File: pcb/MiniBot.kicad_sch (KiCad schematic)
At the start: 39 parts, among them IC1 MMC5633NJL, IC2 MIC23050-SYML-TR, J1 Conn_01x08, J2 Conn_01x02, J3 GSB1C41110SSHR, U1 ESP32-C3-MINI-1-H4X, U3 MCP73832-2-OT

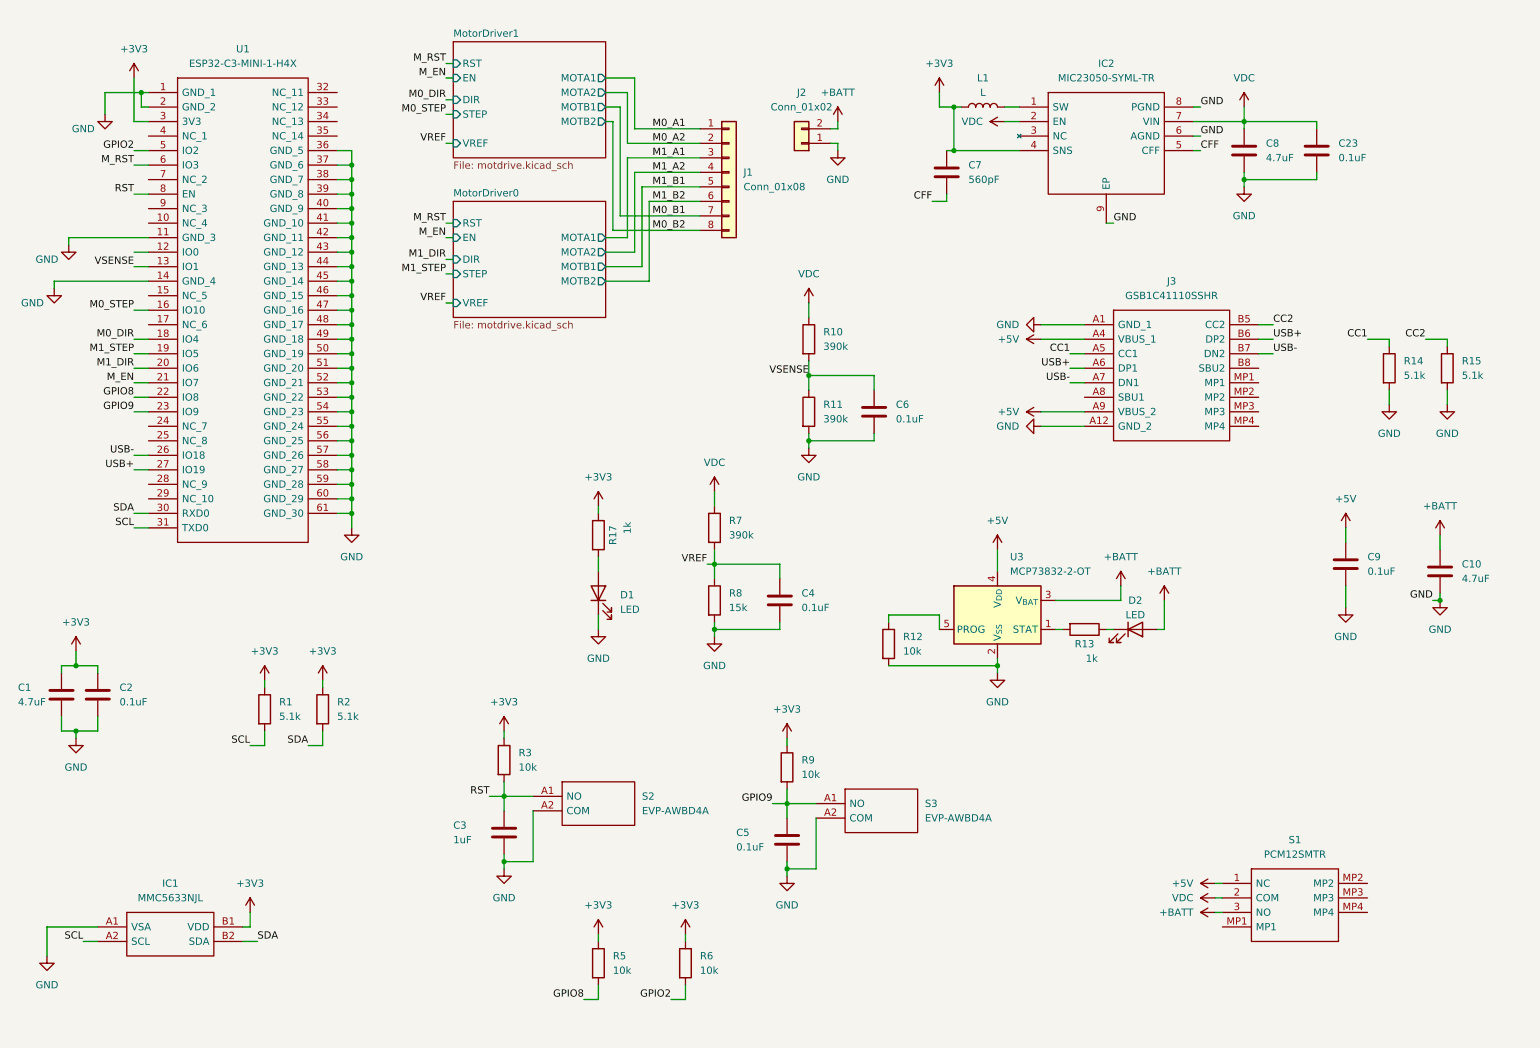
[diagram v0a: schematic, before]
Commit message: getting close to order state
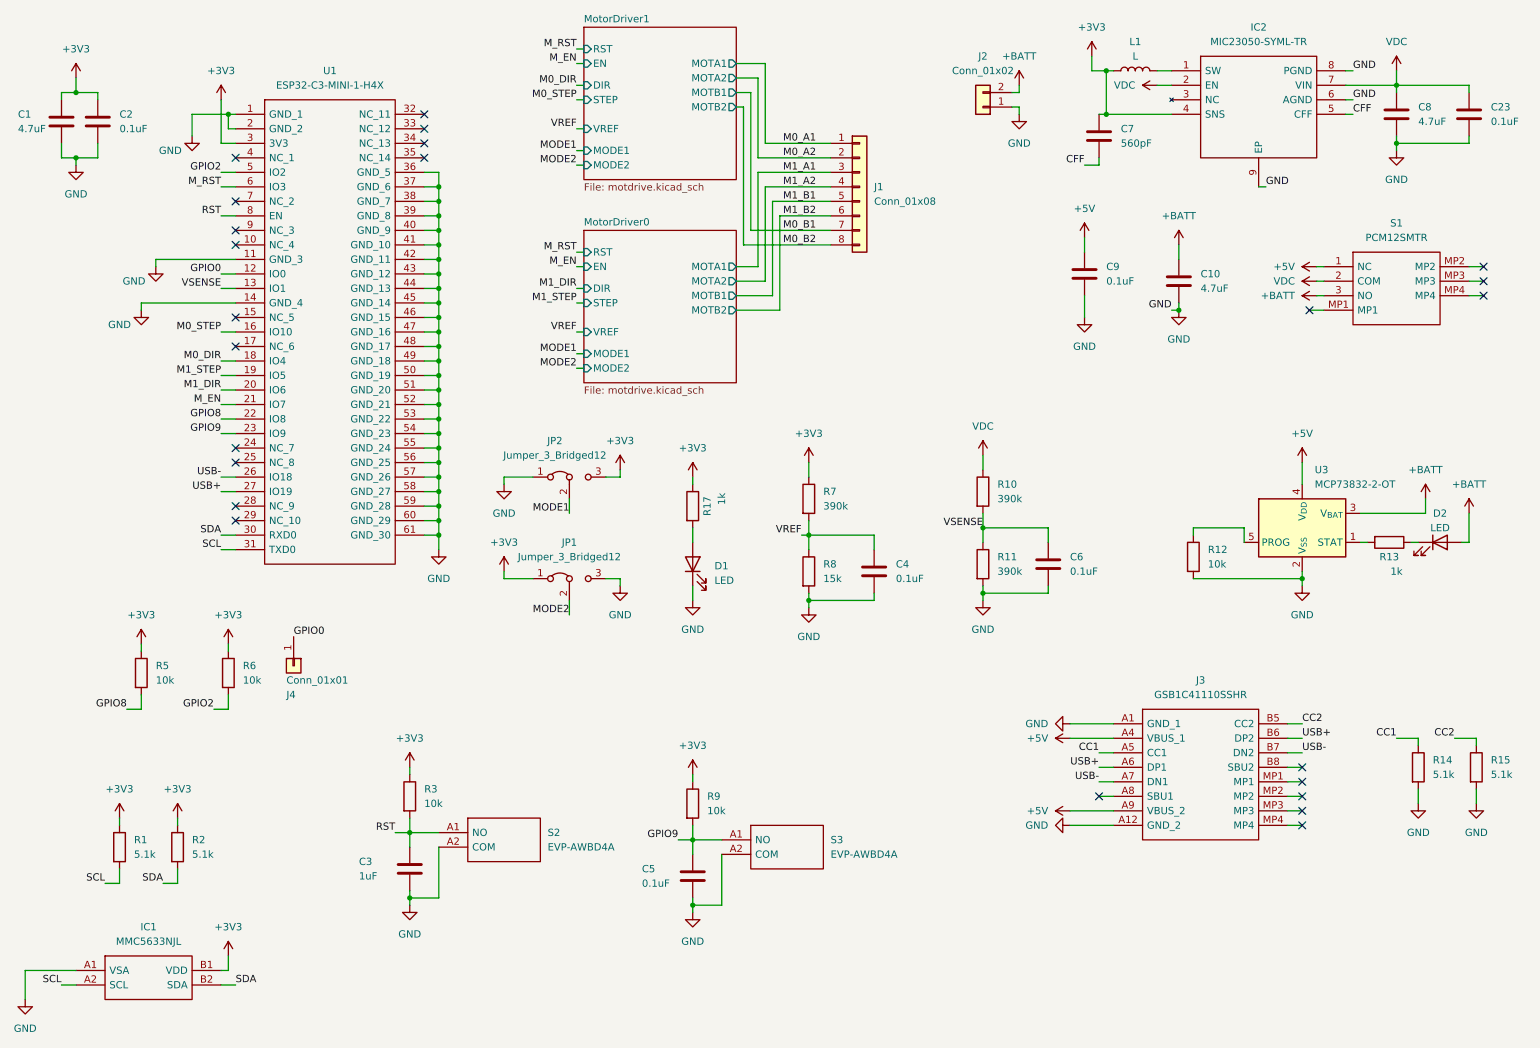
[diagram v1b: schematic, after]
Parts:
- added J4: Conn_01x01, TestPoint:TestPoint_Pad_D1.0mm, symbol Connector_Generic:Conn_01x01
- added JP1, JP2: Jumper_3_Bridged12, Jumper:SolderJumper-3_P1.3mm_Bridged12_RoundedPad1.0x1.5mm, symbol Jumper:Jumper_3_Bridged12
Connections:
- net +3V3: now also R7.1, JP1.1 (A), JP2.3 (B)
- net GND: now also JP1.3 (B), JP2.1 (A)
- net VDC: no longer R7.1
- net GPIO0: now reaches U1.12 (IO0)
- net GPIO0: now also J4.1 (Pin_1)
- new net MODE1: JP2.2 (C)
- new net MODE2: JP1.2 (C)
- no-connect marks 0 -> 24
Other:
- sheet MotorDriver0 ports: added MODE1, MODE2; removed none
- sheet MotorDriver1 ports: added MODE1, MODE2; removed none
- moved on the sheet: C1, C10, C2, C23, C3, C4, C5, C6, C7, C8, C9, D1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
